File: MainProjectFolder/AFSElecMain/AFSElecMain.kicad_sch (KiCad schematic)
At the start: 0 parts

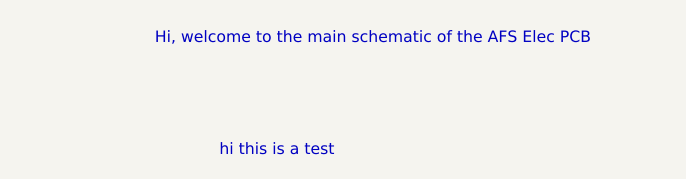
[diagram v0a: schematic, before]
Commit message: hello
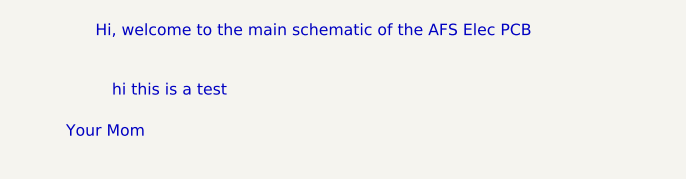
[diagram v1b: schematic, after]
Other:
- note added: "Your Mom"
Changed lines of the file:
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@@
 	(text "hi this is a test"
 		(exclude_from_sim no)
-		(at 50.8 36.576 0)
+		(at 38.862 29.972 0)
+		(effects
+			(font
+				(size 1.27 1.27)
+			)
+		)
+	)
+	(text "Your Mom"
+		(exclude_from_sim no)
+		(at 31.75 34.544 0)
 		(effects
 			(font
@@
 	(text "Hi, welcome to the main schematic of the AFS Elec PCB"
 		(exclude_from_sim no)
-		(at 61.468 24.13 0)
+		(at 54.864 23.368 0)
 		(effects
 			(font
